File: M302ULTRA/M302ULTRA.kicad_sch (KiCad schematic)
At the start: 10 parts, among them J101 XHP8, J102 MID BOARD INTAKE, J103 I2C-1, J104 I2C-2, J105 To Soil Water UNIT, J106 To CO2 UNIT, J107 XHP4, J108 XHP4, J109 XHP4, J110 XHP3

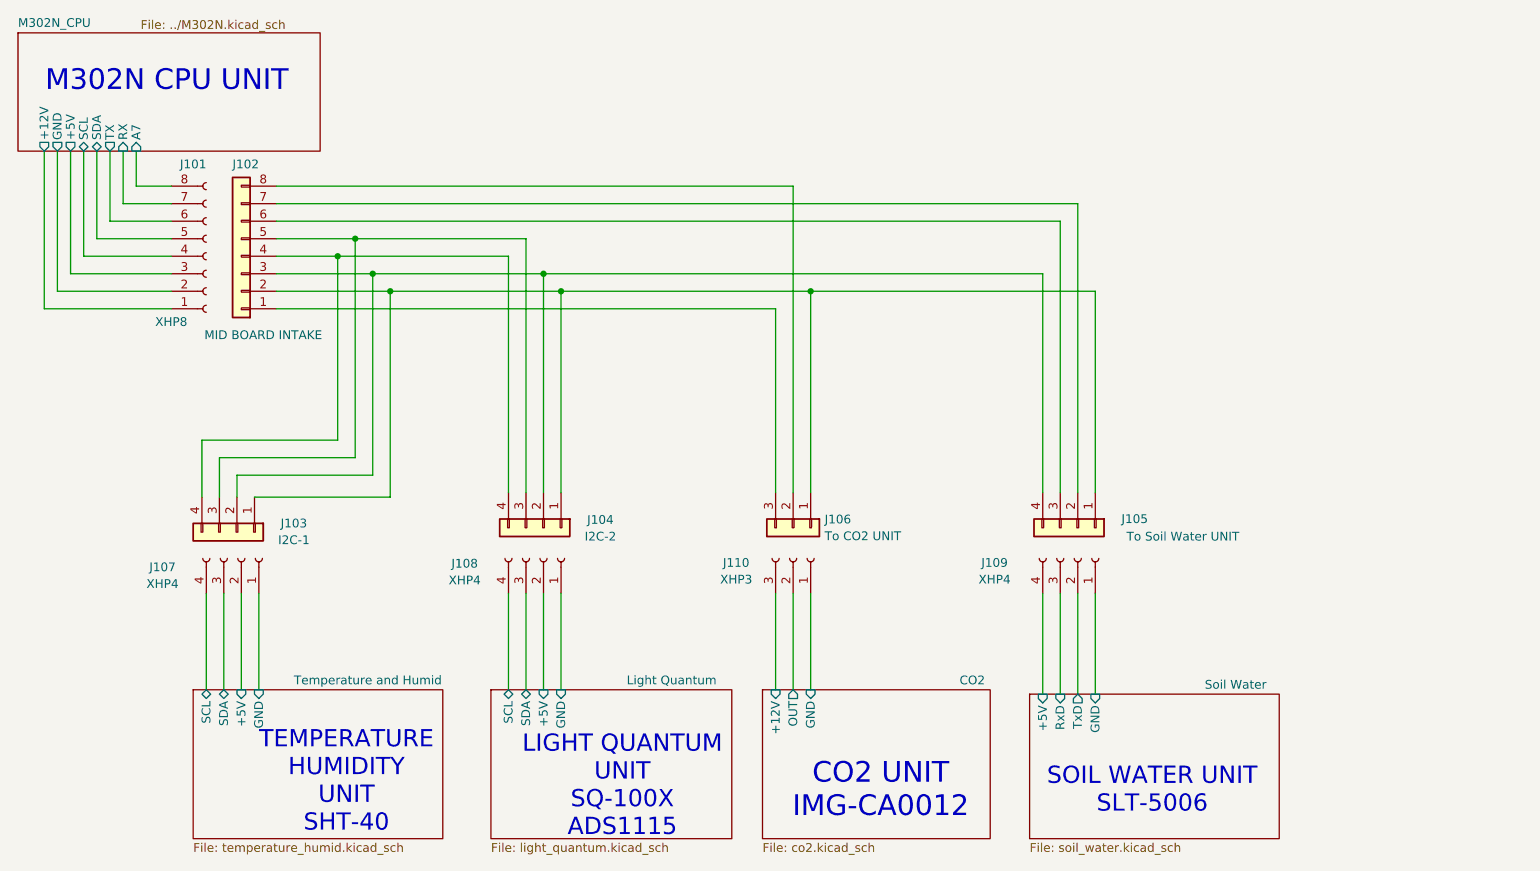
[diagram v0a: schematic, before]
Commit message: ULTRA ver 2.00
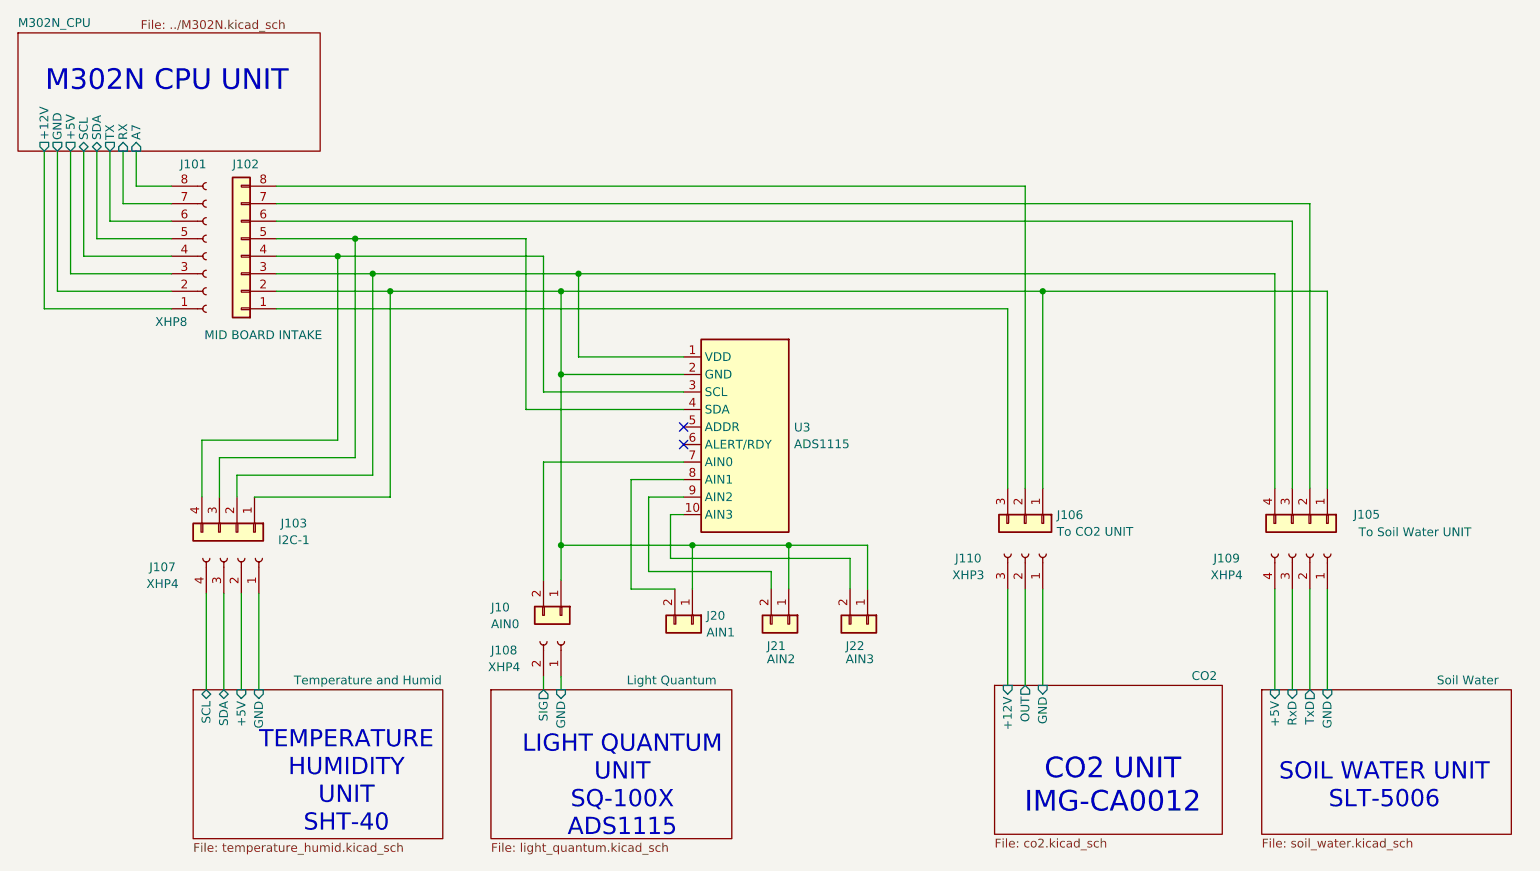
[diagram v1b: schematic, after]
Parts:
- removed J104: I2C-2, symbol Connector_Generic:Conn_01x04
- added J10: AIN0, symbol Connector_Generic:Conn_01x02
- added J20: AIN1, symbol Connector_Generic:Conn_01x02
- added J21: AIN2, symbol Connector_Generic:Conn_01x02
- added J22: AIN3, symbol Connector_Generic:Conn_01x02
- added U3: ADS1115, symbol M302N:ADS1115
- J108: symbol Connector:Conn_01x04_Socket -> Connector:Conn_01x02_Socket
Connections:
- net at J102.2 (Pin_2), J103.1 (Pin_1), J105.1 (Pin_1)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: now also J10.1 (Pin_1), J20.1 (Pin_1), J21.1 (Pin_1), J22.1 (Pin_1), U3.2 (GND)
- net at J102.3 (Pin_3), J103.2 (Pin_2), J105.4 (Pin_4): now also U3.1 (VDD)
- net at J102.4 (Pin_4), J103.4 (Pin_4): now also U3.3 (SCL)
- net at J102.5 (Pin_5), J103.3 (Pin_3): now also U3.4 (SDA)
- net Light Quantum/+5V renamed Light Quantum/SIG
- removed net Light Quantum/SCL: J108.4 (Pin_4)
- removed net Light Quantum/SDA: J108.3 (Pin_3)
- new net: J22.2 (Pin_2), U3.10 (AIN3)
- new net: J10.2 (Pin_2), U3.7 (AIN0)
- new net: J21.2 (Pin_2), U3.9 (AIN2)
- new net: J20.2 (Pin_2), U3.8 (AIN1)
- no-connect marks 0 -> 2
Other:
- sheet Light Quantum ports: added SIG; removed +5V, SCL, SDA
- moved on the sheet: J105, J106, J109, J110
